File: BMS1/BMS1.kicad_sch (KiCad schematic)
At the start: 85 parts, among them U1 LTC6812-1, U2 LTC6812-1, U4325RT1 VTC6, U4325RT10 VTC6, U4325RT11 VTC6, U4325RT12 VTC6, U4325RT13 VTC6, U4325RT14 VTC6, U4325RT15 VTC6, U4325RT16 VTC6, U4325RT17 VTC6, U4325RT18 VTC6, U4325RT19 VTC6, U4325RT2 VTC6, U4325RT20 VTC6, U4325RT21 VTC6, U4325RT22 VTC6, U4325RT23 VTC6, U4325RT24 VTC6, U4325RT25 VTC6, U4325RT3 VTC6, U4325RT4 VTC6, U4325RT5 VTC6, U4325RT6 VTC6, U4325RT7 VTC6, U4325RT8 VTC6, U4325RT9 VTC6

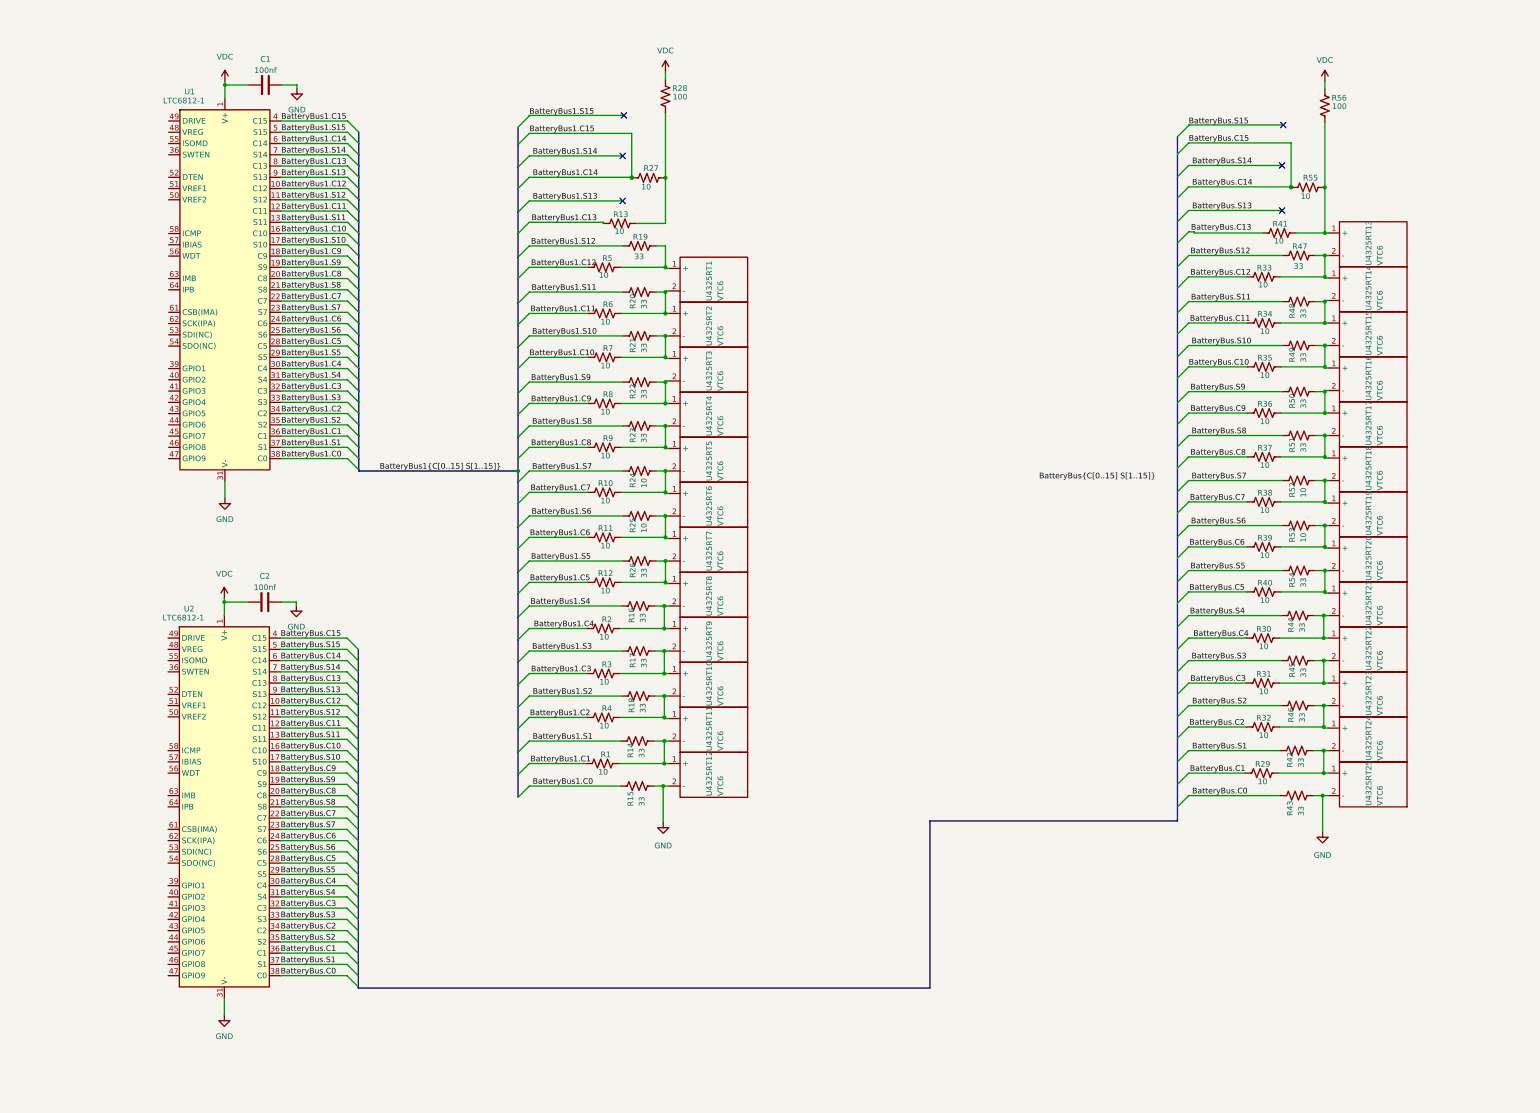
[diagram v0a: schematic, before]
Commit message: sprint 1 push
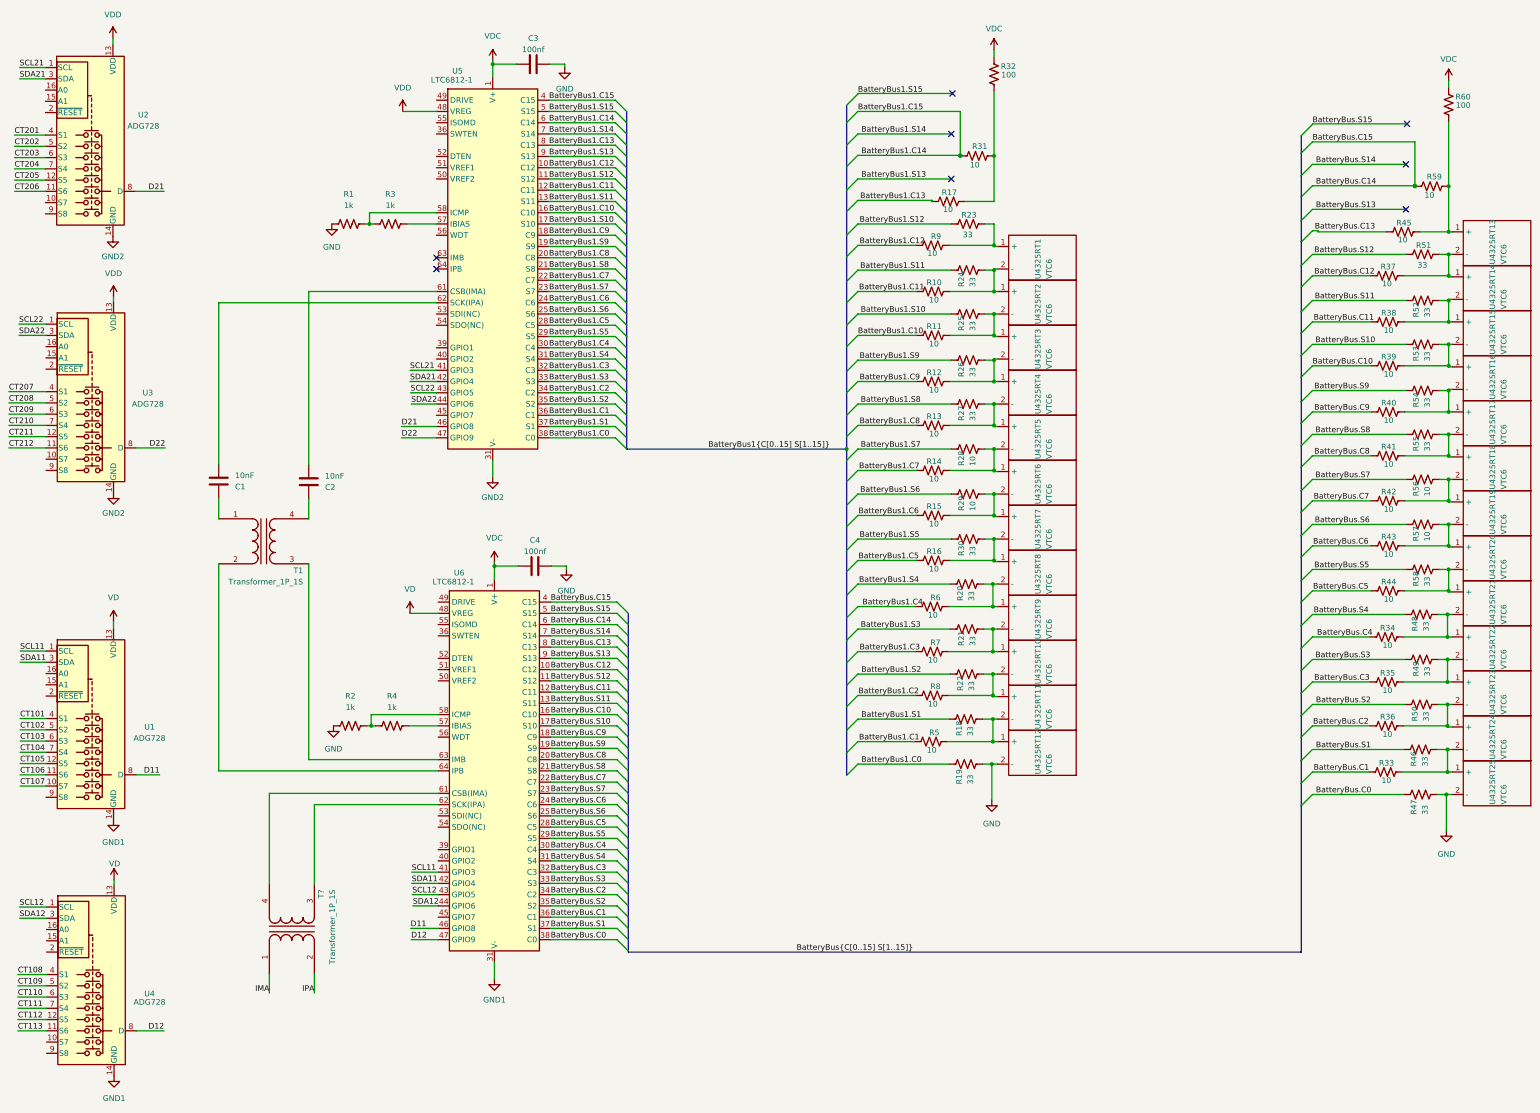
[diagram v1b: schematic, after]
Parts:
- added C1, C2: 10nF, symbol Device:C
- added R1, R2, R3, R4: 1k, symbol Device:R_US
- added T1, T?: Transformer_1P_1S, symbol Device:Transformer_1P_1S
- added U1, U2, U3, U4: ADG728, Package_SO:TSSOP-16_4.4x5mm_P0.65mm, symbol Analog_Switch:ADG728
- renumbered C1 to C3, C2 to C4, R6 to R10, R7 to R11, R8 to R12, R9 to R13, R10 to R14, R11 to R15, R12 to R16, R13 to R17, R14 to R18, R15 to R19, R16 to R20, R17 to R21, R18 to R22, R19 to R23, R20 to R24, R21 to R25, R22 to R26, R23 to R27, R24 to R28, R25 to R29, R26 to R30, R27 to R31, R28 to R32, R29 to R33, R30 to R34, R31 to R35, R32 to R36, R33 to R37, R34 to R38, R35 to R39, R36 to R40, R37 to R41, R38 to R42, R39 to R43, R40 to R44, R41 to R45, R42 to R46, R43 to R47, R44 to R48, R45 to R49, R1 to R5, R46 to R50, R47 to R51, R48 to R52, R49 to R53, R50 to R54, R51 to R55, R52 to R56, R53 to R57, R54 to R58, R55 to R59, R2 to R6, R56 to R60, R3 to R7, R4 to R8, R5 to R9, U1 to U5, U2 to U6
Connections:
- net GND: now also R1.1, R2.1; no longer U5.30 (V-), U5.31 (V-), U5.65 (V-), U6.30 (V-), U6.31 (V-), U6.65 (V-)
- net SCL11: now reaches U6.41 (GPIO3)
- net SCL11: now also U1.1 (SCL)
- net SDA11: now reaches U6.42 (GPIO4)
- net SDA11: now also U1.3 (SDA)
- net SCL12: now reaches U6.43 (GPIO5)
- net SCL12: now also U4.1 (SCL)
- net SDA12: now reaches U6.44 (GPIO6)
- net SDA12: now also U4.3 (SDA)
- net D11: now reaches U6.46 (GPIO8)
- net D11: now also U1.8 (D)
- net D12: now reaches U6.47 (GPIO9)
- net D12: now also U4.8 (D)
- net VD: now reaches U6.48 (VREG)
- net VD: now also U1.13 (VDD), U4.13 (VDD)
- net at U6.57 (IBIAS): now also R4.2
- net at U6.58 (ICMP): now also R2.2, R4.1
- net at U6.61 (CSB(IMA)): now also T?.4 (SB)
- net at U6.62 (SCK(IPA)): now also T?.3 (SA)
- net at U6.63 (IMB): now also T1.3 (SA)
- net at U6.64 (IPB): now also T1.2 (AB)
- net SCL21: now reaches U5.41 (GPIO3)
- net SCL21: now also U2.1 (SCL)
- net SDA21: now reaches U5.42 (GPIO4)
- net SDA21: now also U2.3 (SDA)
- net SCL22: now reaches U5.43 (GPIO5)
- net SCL22: now also U3.1 (SCL)
- net SDA22: now reaches U5.44 (GPIO6)
- net SDA22: now also U3.3 (SDA)
- net D21: now reaches U5.46 (GPIO8)
- net D21: now also U2.8 (D)
- net D22: now reaches U5.47 (GPIO9)
- net D22: now also U3.8 (D)
- net VDD: now reaches U5.48 (VREG)
- net VDD: now also U2.13 (VDD), U3.13 (VDD)
- net at U5.57 (IBIAS): now also R3.2
- net at U5.58 (ICMP): now also R1.2, R3.1
- net at U5.61 (CSB(IMA)): now also C2.1
- net at U5.62 (SCK(IPA)): now also C1.1
- new net: C1.2, T1.1 (AA)
- new net: C2.2, T1.4 (SB)
- new net CT101: U1.4 (S1)
- new net CT102: U1.5 (S2)
- new net CT103: U1.6 (S3)
- new net CT104: U1.7 (S4)
- new net CT105: U1.12 (S5)
- new net CT106: U1.11 (S6)
- new net CT107: U1.10 (S7)
- new net CT108: U4.4 (S1)
- new net CT109: U4.5 (S2)
- new net CT110: U4.6 (S3)
- new net CT111: U4.7 (S4)
- new net CT112: U4.12 (S5)
- new net CT113: U4.11 (S6)
- new net CT201: U2.4 (S1)
- new net CT202: U2.5 (S2)
- new net CT203: U2.6 (S3)
- new net CT204: U2.7 (S4)
- new net CT205: U2.12 (S5)
- new net CT206: U2.11 (S6)
- new net CT207: U3.4 (S1)
- new net CT208: U3.5 (S2)
- new net CT209: U3.6 (S3)
- new net CT210: U3.7 (S4)
- new net CT211: U3.12 (S5)
- new net CT212: U3.11 (S6)
- new net GND1: U1.14 (GND), U4.14 (GND), U6.30 (V-), U6.31 (V-), U6.65 (V-)
- new net GND2: U2.14 (GND), U3.14 (GND), U5.30 (V-), U5.31 (V-), U5.65 (V-)
- new net IMA: T?.1 (AA)
- new net IPA: T?.2 (AB)
- no-connect marks 6 -> 8
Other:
- moved on the sheet: C3, C4, R10, R11, R12, R13, R14, R15, R16, R17, R18, R19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

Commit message: BMS rev1
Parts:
- removed R17, R33, R34: 10, Resistor_SMD:R_1206_3216Metric_Pad1.30x1.75mm_HandSolder, symbol Device:R_US
- removed R32: 100, symbol Device:R_US
- removed T1: Transformer_1P_1S, symbol Device:Transformer_1P_1S
- removed U4325RT1, U4325RT10, U4325RT11, U4325RT12, U4325RT13, U4325RT14, U4325RT15, U4325RT16, U4325RT17, U4325RT18, U4325RT19, U4325RT2, U4325RT20, U4325RT21, U4325RT22, U4325RT23, U4325RT24, U4325RT25, U4325RT3, U4325RT4, U4325RT5, U4325RT6, U4325RT7, U4325RT8, U4325RT9: VTC6, symbol AERO_Symbols:VTC6
- added B1, B10, B11, B12, B13, B14, B15, B16, B17, B18, B19, B2, B20, B21, B22, B23, B24, B25, B3, B4, B5, B6, B7, B8, B9: VTC6+T, symbol AERO_Symbols:VTC6+T
- added C10, C11, C12, C13, C14, C15, C16, C17, C18, C19, C20, C21, C22, C23, C24, C25, C26, C27, C28, C29, C30, C31, C7, C8, C9: 100nF, Capacitor_SMD:C_0603_1608Metric_Pad1.08x0.95mm_HandSolder, symbol Device:C
- added C3, C4: 1uf, Capacitor_SMD:C_0603_1608Metric_Pad1.08x0.95mm_HandSolder, symbol Device:C
- added J1: Conn_01x02, Connector_JST:JST_XH_S2B-XH-A-1_1x02_P2.50mm_Horizontal, symbol Connector_Generic:Conn_01x02
- added R3, R4, R5, R6: 20k, symbol Device:R_US
- added R61: 10, Resistor_SMD:R_1206_3216Metric_Pad1.30x1.75mm_HandSolder, symbol Device:R_US
- added R62: 10, Resistor_SMD:R_0603_1608Metric_Pad0.98x0.95mm_HandSolder, symbol Device:R_US
- added R63, R64, R65, R66, R67, R68, R69, R70, R71, R72, R73, R74, R75: 21, Resistor_SMD:R_0603_1608Metric_Pad0.98x0.95mm_HandSolder, symbol Device:R_US
- added R76: 100, symbol Device:R_US
- added R77, R78, R79, R80, R81, R82, R83, R84, R85, R86, R87, R88, R89: 680, Resistor_SMD:R_0603_1608Metric_Pad0.98x0.95mm_HandSolder, symbol Device:R_US
- added U1, U2, U3, U4: ADG728, Package_SO:TSSOP-16_4.4x5mm_P0.65mm, symbol Analog_Switch:ADG728
- C1, C2: footprint (none) -> Capacitor_SMD:C_0603_1608Metric_Pad1.08x0.95mm_HandSolder
- C5: renamed from C3; footprint (none) -> Capacitor_SMD:C_0603_1608Metric_Pad1.08x0.95mm_HandSolder
- C6: renamed from C4; footprint (none) -> Capacitor_SMD:C_0603_1608Metric_Pad1.08x0.95mm_HandSolder
- R1: footprint (none) -> Resistor_SMD:R_2512_6332Metric_Pad1.40x3.35mm_HandSolder
- R10: renamed from R19; value 33 -> 10
- R23: renamed from R24; value 33 -> 21; footprint Resistor_SMD:R_0603_1608Metric_Pad0.98x0.95mm_HandSolder -> Resistor_SMD:R_2512_6332Metric_Pad1.40x3.35mm_HandSolder
- R24: renamed from R20; value 33 -> 21; footprint Resistor_SMD:R_0603_1608Metric_Pad0.98x0.95mm_HandSolder -> Resistor_SMD:R_2512_6332Metric_Pad1.40x3.35mm_HandSolder
- R25: renamed from R18; value 33 -> 21; footprint Resistor_SMD:R_0603_1608Metric_Pad0.98x0.95mm_HandSolder -> Resistor_SMD:R_2512_6332Metric_Pad1.40x3.35mm_HandSolder
- R26: renamed from R25; value 33 -> 21; footprint Resistor_SMD:R_0603_1608Metric_Pad0.98x0.95mm_HandSolder -> Resistor_SMD:R_2512_6332Metric_Pad1.40x3.35mm_HandSolder
- R27: renamed from R30; value 33 -> 21; footprint Resistor_SMD:R_0603_1608Metric_Pad0.98x0.95mm_HandSolder -> Resistor_SMD:R_2512_6332Metric_Pad1.40x3.35mm_HandSolder
- R28: renamed from R23; value 33 -> 21; footprint Resistor_SMD:R_0603_1608Metric_Pad0.98x0.95mm_HandSolder -> Resistor_SMD:R_2512_6332Metric_Pad1.40x3.35mm_HandSolder
- R29: renamed from R26; value 33 -> 21; footprint Resistor_SMD:R_0603_1608Metric_Pad0.98x0.95mm_HandSolder -> Resistor_SMD:R_2512_6332Metric_Pad1.40x3.35mm_HandSolder
- R30: renamed from R27; value 33 -> 21; footprint Resistor_SMD:R_0603_1608Metric_Pad0.98x0.95mm_HandSolder -> Resistor_SMD:R_2512_6332Metric_Pad1.40x3.35mm_HandSolder
- R31: renamed from R22; value 33 -> 21; footprint Resistor_SMD:R_0603_1608Metric_Pad0.98x0.95mm_HandSolder -> Resistor_SMD:R_2512_6332Metric_Pad1.40x3.35mm_HandSolder
- R32: renamed from R28; value 10 -> 21; footprint Resistor_SMD:R_0603_1608Metric_Pad0.98x0.95mm_HandSolder -> Resistor_SMD:R_2512_6332Metric_Pad1.40x3.35mm_HandSolder
- R33: renamed from R21; value 33 -> 21; footprint Resistor_SMD:R_0603_1608Metric_Pad0.98x0.95mm_HandSolder -> Resistor_SMD:R_2512_6332Metric_Pad1.40x3.35mm_HandSolder
- R34: renamed from R29; value 10 -> 21; footprint Resistor_SMD:R_0603_1608Metric_Pad0.98x0.95mm_HandSolder -> Resistor_SMD:R_2512_6332Metric_Pad1.40x3.35mm_HandSolder
- R35: value 10 -> 100; footprint Resistor_SMD:R_1206_3216Metric_Pad1.30x1.75mm_HandSolder -> (none)
- R36, R37, R38, R39, R40, R41, R42, R43, R44, R45: value 10 -> 680; footprint Resistor_SMD:R_1206_3216Metric_Pad1.30x1.75mm_HandSolder -> Resistor_SMD:R_0603_1608Metric_Pad0.98x0.95mm_HandSolder
- R46, R47: value 33 -> 680
- R48, R49, R51, R52, R53, R54, R55, R58: value 33 -> 10; footprint Resistor_SMD:R_0603_1608Metric_Pad0.98x0.95mm_HandSolder -> Resistor_SMD:R_1206_3216Metric_Pad1.30x1.75mm_HandSolder
- R50: value 33 -> 100
- R56, R57: footprint Resistor_SMD:R_0603_1608Metric_Pad0.98x0.95mm_HandSolder -> Resistor_SMD:R_1206_3216Metric_Pad1.30x1.75mm_HandSolder
- R59: footprint (none) -> Resistor_SMD:R_1206_3216Metric_Pad1.30x1.75mm_HandSolder
- R60: value 100 -> 10; footprint (none) -> Resistor_SMD:R_1206_3216Metric_Pad1.30x1.75mm_HandSolder
- R9: renamed from R31; value 10 -> 100
- U10: renamed from U6; footprint (none) -> AERO_Footprints:QFP-64_11x11_Pitch0.5mm
- U9: renamed from U5; footprint (none) -> AERO_Footprints:QFP-64_11x11_Pitch0.5mm
- gave numbers to parts that had none: 1
- renumbered R6 to R11, R5 to R12, R10 to R13, R11 to R14, R8 to R15, R9 to R16, R16 to R17, R7 to R18, R12 to R19, R13 to R20, R14 to R21, R15 to R22, R3 to R7, R4 to R8, U2 to U5, U3 to U6, U1 to U7, U4 to U8
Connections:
- net BatteryBus1.C14 is gone; now on net BatteryBus1.C13: R9.1, U9.4 (C15), U9.6 (C14)
- net BatteryBus.C0: now also R62.2; no longer R47.2
- net BatteryBus.C1: now also R49.2, C31.1
- net BatteryBus.C10: now also R52.2, C22.1; no longer R39.2
- net BatteryBus.C11: now also R51.2, C21.1; no longer R38.2
- net BatteryBus.C12: now also R55.2, C20.1; no longer R37.2
- net BatteryBus.C13: now also R54.2, C19.1; no longer R45.2
- net BatteryBus.C14: now also R50.1; no longer R59.1
- net BatteryBus.C2: now also R53.2, C30.1; no longer R36.2
- net BatteryBus.C3: now also R57.2, C29.1; no longer R35.2
- net BatteryBus.C4: now also R48.2, C28.1
- net BatteryBus.C5: now also R56.2, C27.1; no longer R44.2
- net BatteryBus.C6: now also C26.1, R61.2; no longer R43.2
- net BatteryBus.C7: now also R60.2, C25.1; no longer R42.2
- net BatteryBus.C8: now also R59.2, C24.1; no longer R41.2
- net BatteryBus.C9: now also R58.2, C23.1; no longer R40.2
- net BatteryBus.S1: now also R65.2; no longer R46.2
- net BatteryBus.S10: now also R66.2; no longer R53.2
- net BatteryBus.S11: now also R63.2; no longer R52.2
- net BatteryBus.S12: now also R68.2; no longer R51.2
- net BatteryBus.S13: now also R75.2
- net BatteryBus.S2: now also R71.2; no longer R50.2
- net BatteryBus.S3: now also R73.2; no longer R49.2
- net BatteryBus.S4: now also R64.2; no longer R48.2
- net BatteryBus.S5: now also R67.2; no longer R58.2
- net BatteryBus.S6: now also R74.2; no longer R57.2
- net BatteryBus.S7: now also R72.2; no longer R56.2
- net BatteryBus.S8: now also R70.2; no longer R55.2
- net BatteryBus.S9: now also R69.2; no longer R54.2
- net BatteryBus1.C1: now also C18.1
- net BatteryBus1.C10: now also C9.1
- net BatteryBus1.C11: now also C8.1
- net BatteryBus1.C12: now also C7.1
- net BatteryBus1.C2: now also C17.1
- net BatteryBus1.C3: now also C16.1
- net BatteryBus1.C4: now also C15.1
- net BatteryBus1.C5: now also C14.1
- net BatteryBus1.C6: now also C13.1
- net BatteryBus1.C7: now also C12.1
- net BatteryBus1.C8: now also C11.1
- net BatteryBus1.C9: now also C10.1
- net CT101: now also B25.3 (T+), R89.1
- net CT102: now also B24.3 (T+), R88.1
- net CT103: now also B23.3 (T+), R87.1
- net CT104: now also B22.3 (T+), R86.1
- net CT105: now also B21.3 (T+), R85.1
- net CT106: now also B20.3 (T+), R84.1
- net CT107: now also B19.3 (T+), R83.1
- net CT108: now also B18.3 (T+), R82.1
- net CT109: now also B17.3 (T+), R81.1
- net CT110: now also B16.3 (T+), R80.1
- net CT111: now also B15.3 (T+), R79.1
- net CT112: now also B14.3 (T+), R78.1
- net CT113: now also B13.3 (T+), R77.1
- net CT201: now also R47.1, B12.3 (T+)
- net CT202: now also R46.1, B11.3 (T+)
- net CT203: now also R45.1, B10.3 (T+)
- net CT204: now also R44.1, B9.3 (T+)
- net CT205: now also R43.1, B8.3 (T+)
- net CT206: now also R42.1, B7.3 (T+)
- net CT207: now also R41.1, B6.3 (T+)
- net CT208: now also R40.1, B5.3 (T+)
- net CT209: now also R39.1, B4.3 (T+)
- net CT210: now also R38.1, B3.3 (T+)
- net CT211: now also R37.1, B2.3 (T+)
- net CT212: now also R36.1, B1.3 (T+)
- net GND: now also C10.2, C11.2, C12.2, C13.2, C14.2, C15.2, C16.2, C17.2, C18.2, C19.2, C20.2, C21.2, C22.2, C23.2, C24.2, C25.2, C26.2, C27.2, C28.2, C29.2, C30.2, C31.2, C7.2, C8.2, C9.2; no longer R1.1, R10.1, R2.1, R47.1
- net GND1: now also R2.1, U10.59 (V-), U10.60 (V-), U7.16 (A0), B13.4 (T-), B14.4 (T-), B15.4 (T-), B16.4 (T-), B17.4 (T-), B18.4 (T-), B19.4 (T-), B20.4 (T-), B21.4 (T-), B22.4 (T-), B23.4 (T-), B24.4 (T-), B25.2 (-), B25.4 (T-), C3.1, R62.1, U3.14 (GND), U4.14 (GND), U4.16 (A0); no longer U10.30 (V-), U10.31 (V-)
- net GND2: now also R1.1, R10.1, U5.16 (A0), U9.59 (V-), U9.60 (V-), B1.4 (T-), B10.4 (T-), B11.4 (T-), B12.2 (-), B12.4 (T-), B2.4 (T-), B3.4 (T-), B4.4 (T-), B5.4 (T-), B6.4 (T-), B7.4 (T-), B8.4 (T-), B9.4 (T-), C4.1, U1.14 (GND), U1.16 (A0), U2.14 (GND); no longer U9.30 (V-), U9.31 (V-)
- net IMA: now also J1.2 (Pin_2)
- net IPA: now also J1.1 (Pin_1)
- net VD: now also U10.55 (ISOMD), U7.15 (A1), U7.2 (~{RESET}), U8.15 (A1), U8.16 (A0), U8.2 (~{RESET}), R5.1, R6.1, U3.13 (VDD), U3.15 (A1), U3.16 (A0), U3.2 (~{RESET}), U3.8 (D), U4.13 (VDD), U4.15 (A1), U4.2 (~{RESET}), U4.8 (D)
- net VDC: now also R35.1, R3.1, R4.1; no longer C6.1, R60.1, U10.1 (V+)
- net VDD: now also U5.15 (A1), U5.2 (~{RESET}), U6.15 (A1), U6.16 (A0), U6.2 (~{RESET}), U9.55 (ISOMD), U1.13 (VDD), U1.15 (A1), U1.2 (~{RESET}), U1.8 (D), U2.13 (VDD), U2.15 (A1), U2.16 (A0), U2.2 (~{RESET}), U2.8 (D)
- net at R11.1, R24.1: now also B8.2 (-), B9.1 (+)
- net at R18.1, R33.1: now also B10.1 (+), B9.2 (-)
- net at R20.1, R30.1: now also B4.2 (-), B5.1 (+)
- net at R21.1, R32.1: now also B5.2 (-), B6.1 (+)
- net at R15.1, R31.1: now also B10.2 (-), B11.1 (+)
- net at R54.1: now also R50.2, B13.1 (+), R75.1, R76.2; no longer R40.1
- net at R12.1, R25.1: now also B11.2 (-), B12.1 (+)
- net at R13.1, R23.1: now also B1.2 (-), B2.1 (+)
- net at R55.1: now also B13.2 (-), B14.1 (+), R68.1; no longer R41.1
- net at C1.2: now also U10.64 (IPB)
- net at R14.1, R26.1: now also B2.2 (-), B3.1 (+)
- net at R19.1, R29.1: now also B3.2 (-), B4.1 (+)
- net at R16.1, R28.1: now also R35.2, R9.2, B1.1 (+)
- net at U10.63 (IMB): now also C2.2
- net at R17.1, R27.1: now also B7.2 (-), B8.1 (+)
- net at R49.1: now also B24.2 (-), B25.1 (+), R65.1; no longer R35.1
- net at R53.1: now also B23.2 (-), B24.1 (+), R71.1; no longer R39.1
- net at U10.51 (VREF1): now also C3.2
- net at R58.1: now also B16.2 (-), B17.1 (+), R69.1; no longer R44.1
- net at R22.1, R34.1: now also B6.2 (-), B7.1 (+)
- net at R51.1: now also B14.2 (-), B15.1 (+), R63.1; no longer R37.1
- net at R52.1: now also B15.2 (-), B16.1 (+), R66.1; no longer R38.1
- net at R48.1: now also B21.2 (-), B22.1 (+), R64.1
- net at R56.1: now also B20.2 (-), B21.1 (+), R67.1; no longer R42.1
- net at R57.1: now also B22.2 (-), B23.1 (+), R73.1; no longer R43.1
- net at U9.51 (VREF1): now also C4.2
- net SCL11 renamed SCL1
- net SCL1: now also U8.1 (SCL), R5.2, U3.1 (SCL), U4.1 (SCL)
- net SCL12: no longer names the net of U10.43 (GPIO5)
- net SCL12: no longer U8.1 (SCL)
- net SCL21 renamed SCL2
- net SCL2: now also U6.1 (SCL), R3.2, U1.1 (SCL), U2.1 (SCL)
- net SCL22: no longer names the net of U9.43 (GPIO5)
- net SCL22: no longer U6.1 (SCL)
- net SDA11 renamed SDA1
- net SDA1: now also U8.3 (SDA), R6.2, U3.3 (SDA), U4.3 (SDA)
- net SDA12: no longer names the net of U10.44 (GPIO6)
- net SDA12: no longer U8.3 (SDA)
- net SDA21 renamed SDA2
- net SDA2: now also U6.3 (SDA), R4.2, U1.3 (SDA), U2.3 (SDA)
- net SDA22: no longer names the net of U9.44 (GPIO6)
- net SDA22: no longer U6.3 (SDA)
- new net: B18.2 (-), B19.1 (+), R60.1, R72.1
- new net: B19.2 (-), B20.1 (+), R61.1, R74.1
- new net: B17.2 (-), B18.1 (+), R59.1, R70.1
- new net C+101: R89.2, U4.4 (S1)
- new net C+102: R88.2, U4.5 (S2)
- new net C+103: R87.2, U4.6 (S3)
- new net C+104: R86.2, U4.7 (S4)
- new net C+105: R85.2, U4.12 (S5)
- new net C+106: R84.2, U4.11 (S6)
- new net C+107: R83.2, U4.10 (S7)
- new net C+108: R82.2, U3.4 (S1)
- new net C+109: R81.2, U3.5 (S2)
- new net C+110: R80.2, U3.6 (S3)
- new net C+111: R79.2, U3.7 (S4)
- new net C+112: R78.2, U3.12 (S5)
- new net C+113: R77.2, U3.11 (S6)
- new net C+201: R47.2, U1.4 (S1)
- new net C+202: R46.2, U1.5 (S2)
- new net C+203: R45.2, U1.6 (S3)
- new net C+204: R44.2, U1.7 (S4)
- new net C+205: R43.2, U1.12 (S5)
- new net C+206: R42.2, U1.11 (S6)
- new net C+207: R41.2, U2.4 (S1)
- new net C+208: R40.2, U2.5 (S2)
- new net C+209: R39.2, U2.6 (S3)
- new net C+210: R38.2, U2.7 (S4)
- new net C+211: R37.2, U2.12 (S5)
- new net C+212: R36.2, U2.11 (S6)
- new net VCC: C6.1, R76.1, U10.1 (V+)
- no-connect marks 8 -> 35
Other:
- note added: "Mux set 1"
- note added: "Mux set 2"
- note added: "Mux set 3"
- note added: "Mux set 4"
- note added: "Temp sensor MUX Stack 1"
- note added: "Temp sensor MUX Stack 2"
- moved on the sheet: C1, C2, C5, C6, R1, R10, R11, R12, R13, R14, R15, R16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

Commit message: start footprint
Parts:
- B1, B10, B11, B12, B13, B14, B15, B16, B17, B18, B19, B2, B20, B21, B22, B23, B24, B25, B3, B4, B5, B6, B7, B8, B9: footprint (none) -> AERO_Footprints:VTC-6
